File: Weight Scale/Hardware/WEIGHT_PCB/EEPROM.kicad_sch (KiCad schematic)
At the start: 1 part, among them IC3 AT24C04C-SSHM-T

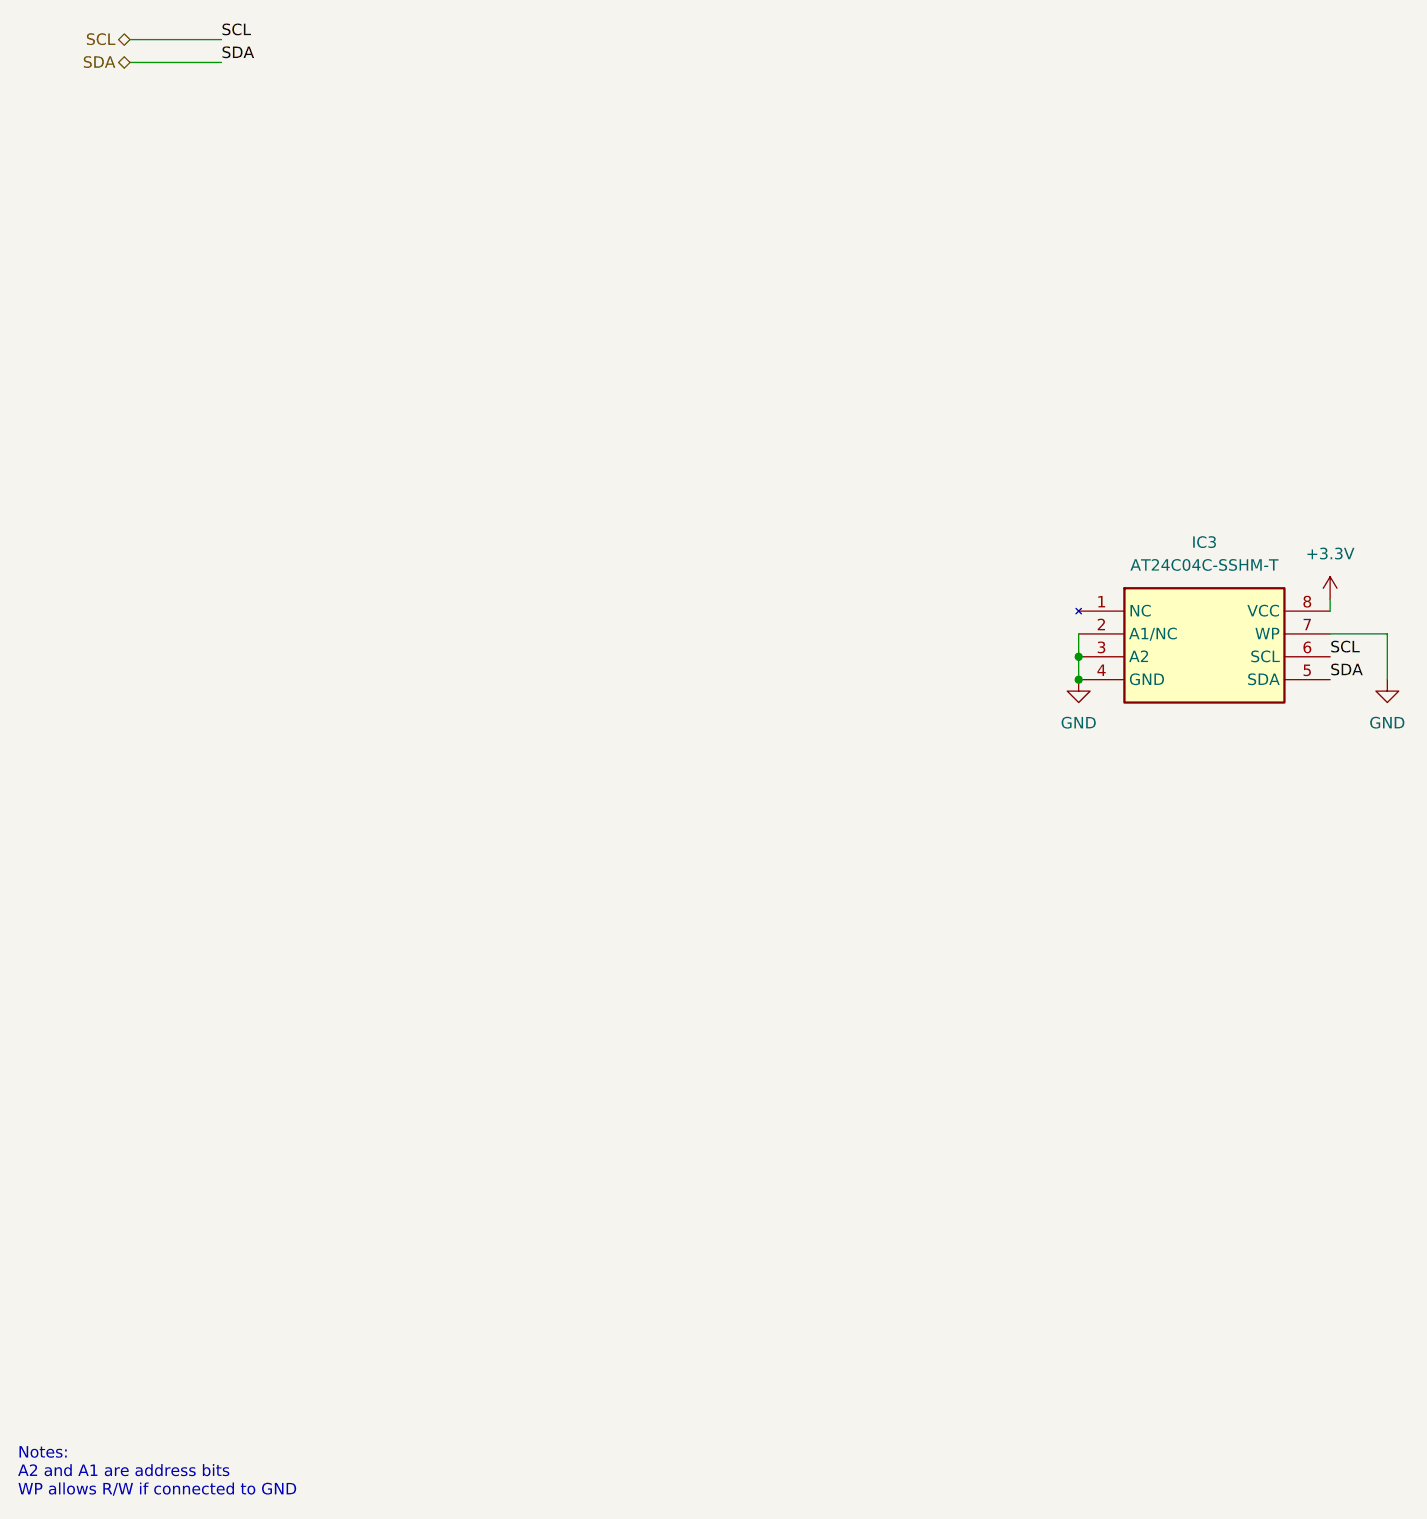
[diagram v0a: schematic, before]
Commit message: update schematics
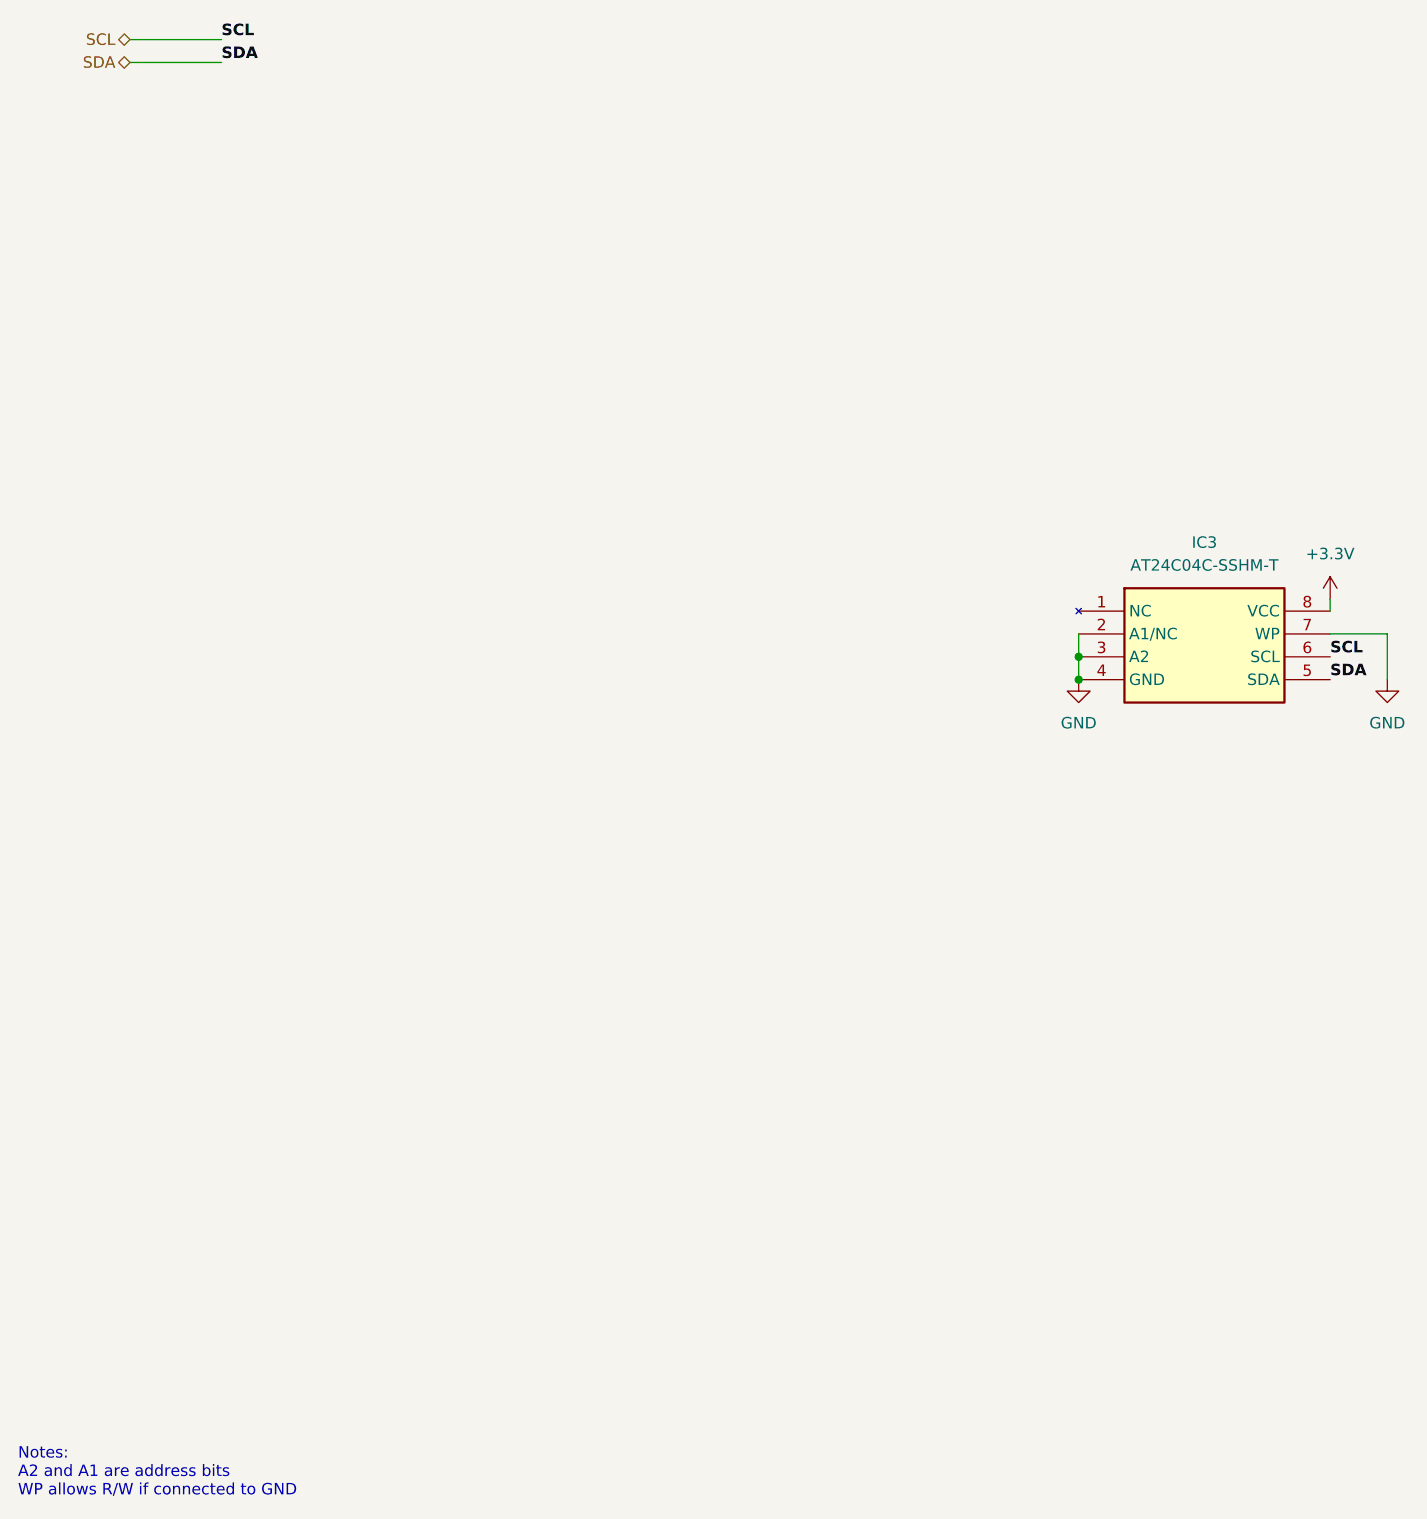
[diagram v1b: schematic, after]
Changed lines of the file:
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@@
 			(font
 				(size 1.27 1.27)
+				(bold yes)
 			)
 			(justify left bottom)
@@
 			(font
 				(size 1.27 1.27)
+				(bold yes)
 			)
 			(justify left bottom)
@@
 			(font
 				(size 1.27 1.27)
+				(bold yes)
 			)
 			(justify left bottom)
@@
 			(font
 				(size 1.27 1.27)
+				(bold yes)
 			)
 			(justify left bottom)

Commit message: update schematics
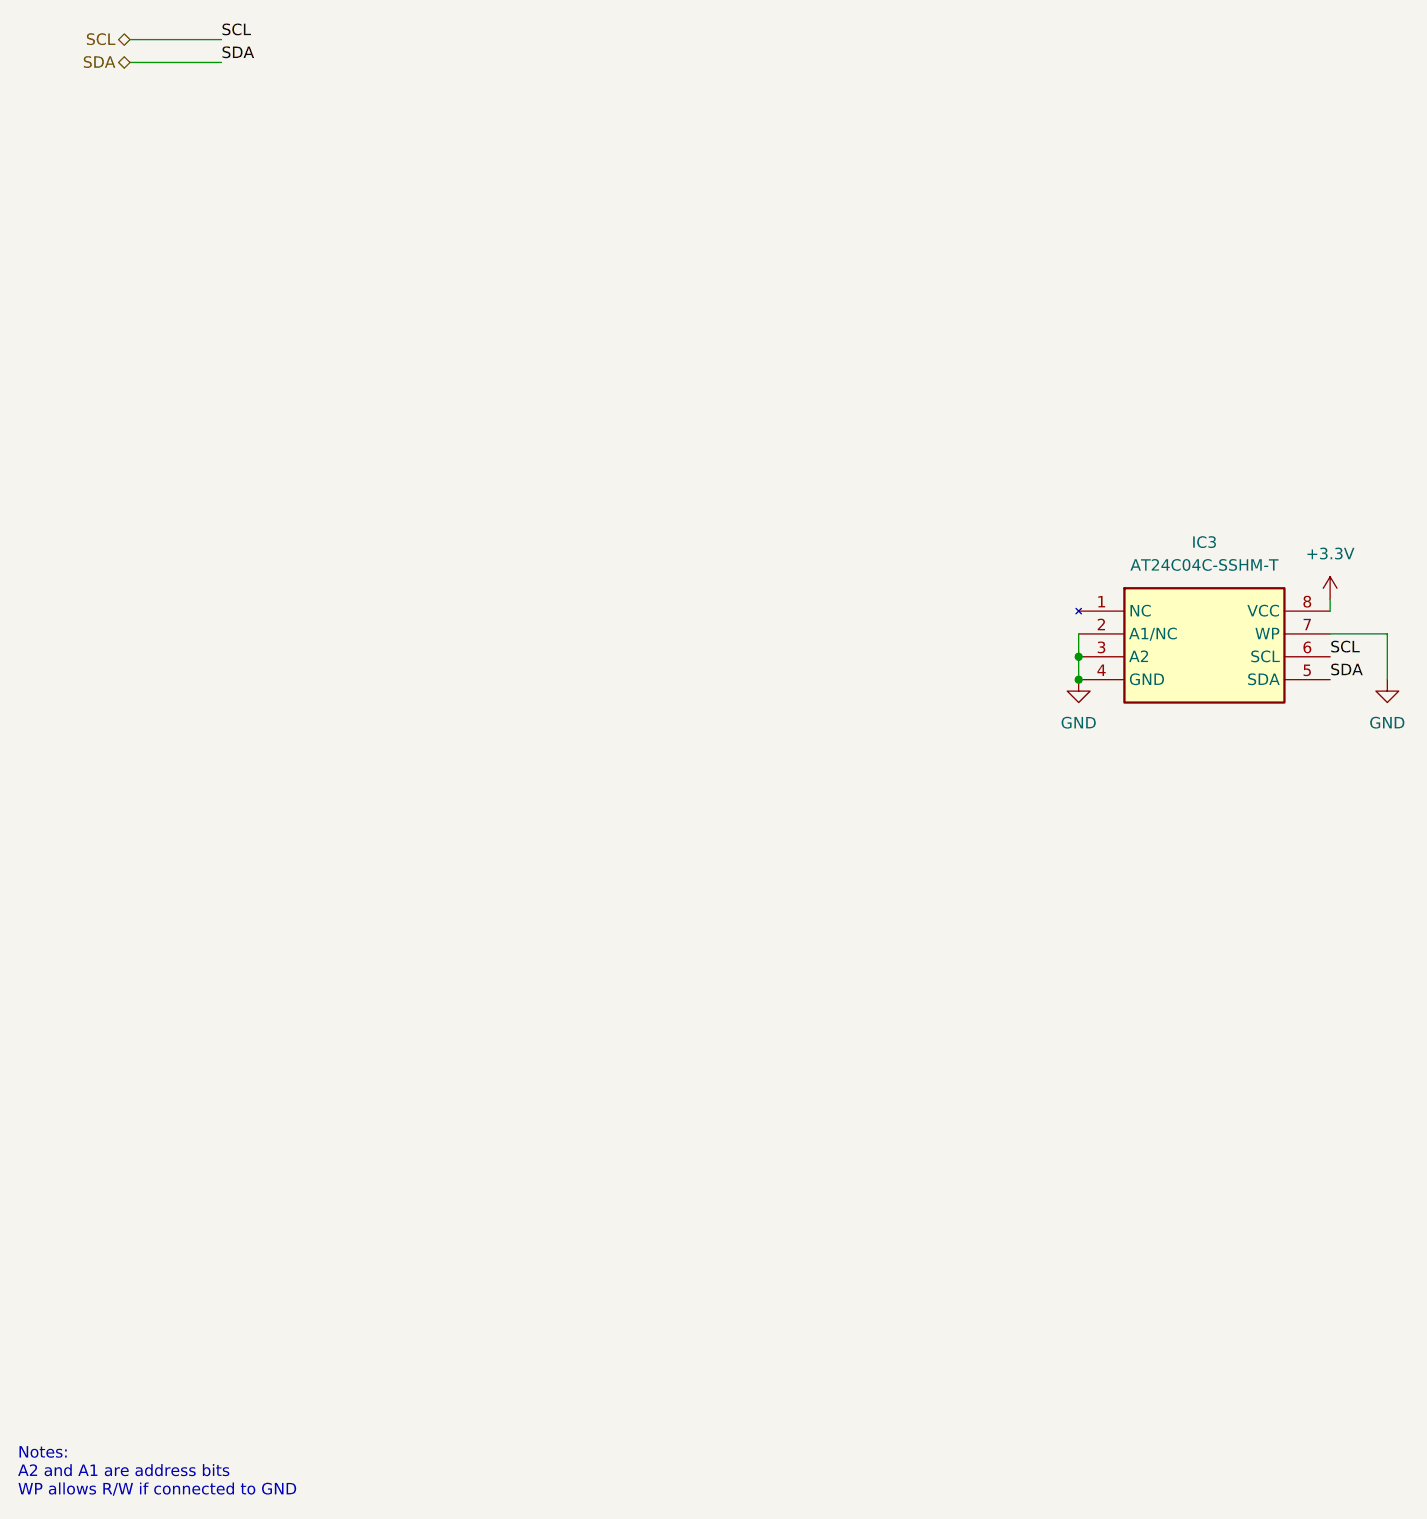
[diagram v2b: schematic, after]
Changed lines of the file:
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@@
 			(font
 				(size 1.27 1.27)
-				(bold yes)
+				(thickness 0.1588)
 			)
 			(justify left bottom)
@@
 			(font
 				(size 1.27 1.27)
-				(bold yes)
+				(thickness 0.1588)
 			)
 			(justify left bottom)
@@
 			(font
 				(size 1.27 1.27)
-				(bold yes)
+				(thickness 0.1588)
 			)
 			(justify left bottom)
@@
 			(font
 				(size 1.27 1.27)
-				(bold yes)
+				(thickness 0.1588)
 			)
 			(justify left bottom)
